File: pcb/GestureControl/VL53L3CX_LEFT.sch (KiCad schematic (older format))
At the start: 25 parts, among them U11 VL53L3CXV0DH_LEFT, U5 VL53L3CXV0DH_LEFT, U9 VL53L3CXV0DH_LEFT

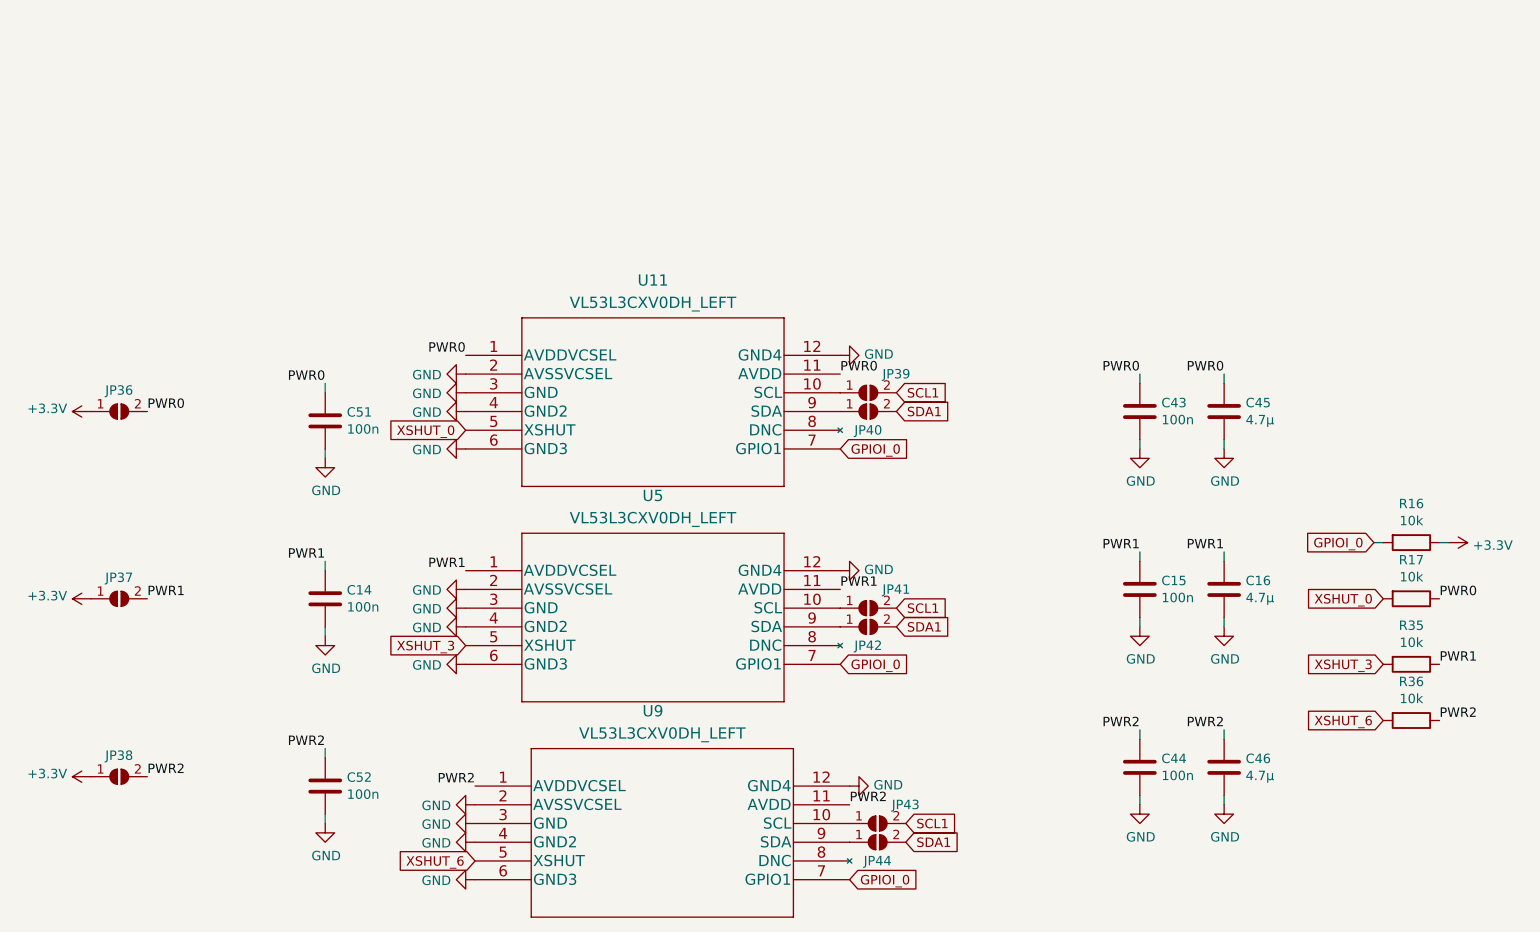
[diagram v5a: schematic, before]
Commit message: add PCB V12
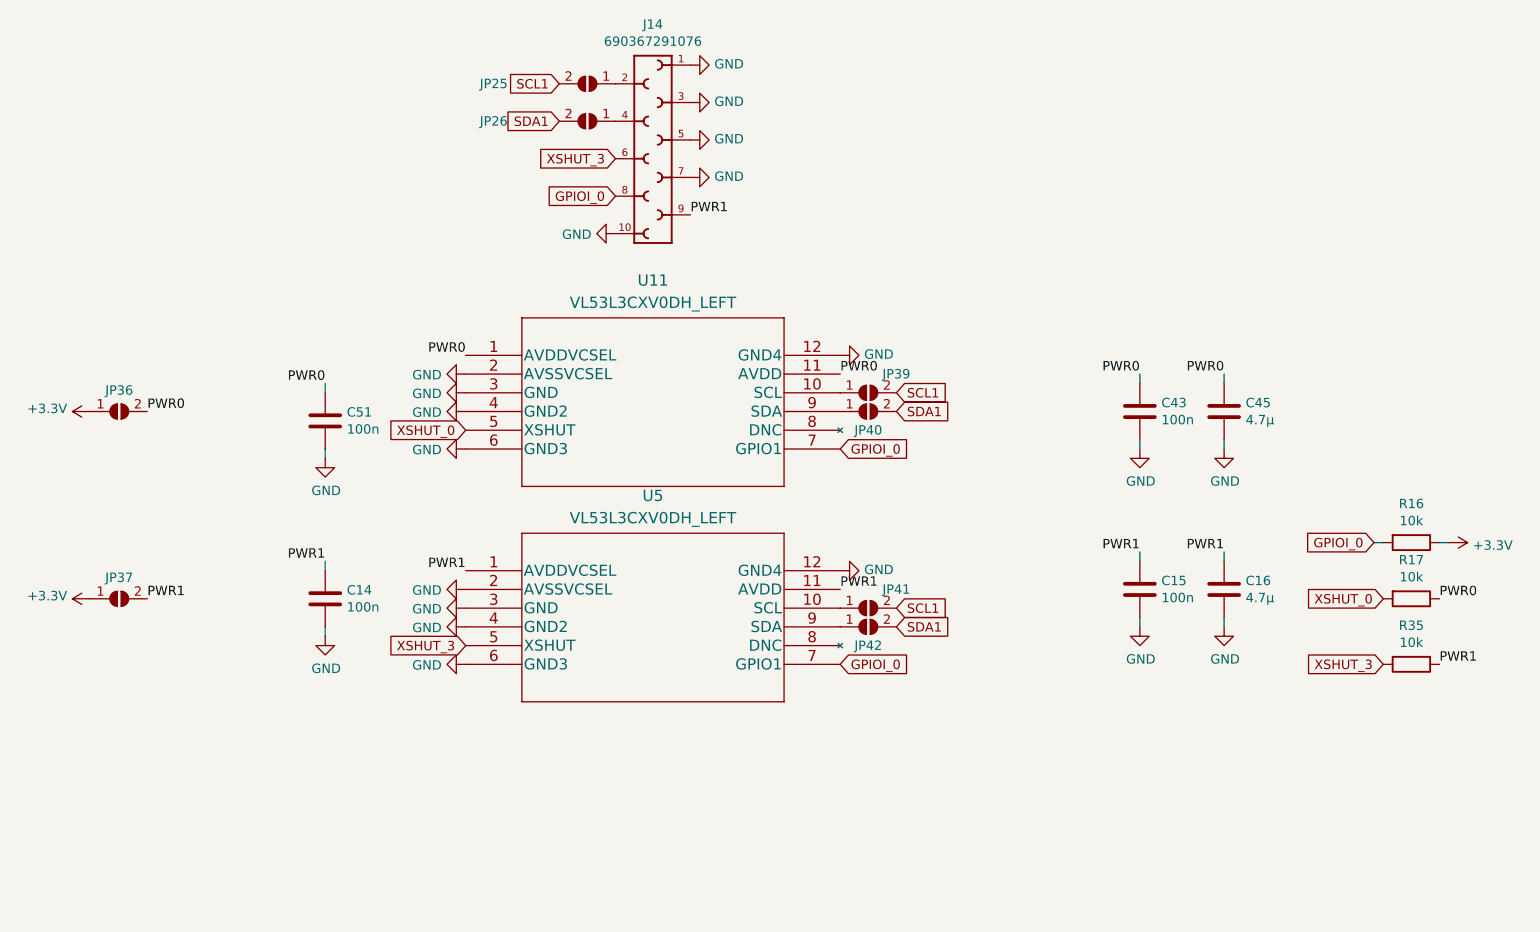
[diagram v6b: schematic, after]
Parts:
- removed C44, C52: 100n, Capacitor_SMD:C_0603_1608Metric_Pad1.08x0.95mm_HandSolder, symbol Device:C
- removed C46: 4.7µ, Capacitor_SMD:C_0805_2012Metric_Pad1.18x1.45mm_HandSolder, symbol Device:C
- removed JP38, JP43, JP44: SolderJumper_2_Open, Jumper:SolderJumper-2_P1.3mm_Open_Pad1.0x1.5mm, symbol Jumper:SolderJumper_2_Open
- removed R36: 10k, Resistor_SMD:R_0805_2012Metric_Pad1.20x1.40mm_HandSolder, symbol Device:R
- removed U9: VL53L3CXV0DH_LEFT, VL53L3CX:VL53L3CXV0DH&slash_1, symbol VL53L3CX:VL53L3CXV0DH_1
- added J14: 690367291076, WR-MM Female SMT Connector:WR-MM Female SMT Connector, symbol WR-MM_Female_SMT_Connector:690367291076
- added JP25, JP26: SolderJumper_2_Open, Jumper:SolderJumper-2_P1.3mm_Open_Pad1.0x1.5mm, symbol Jumper:SolderJumper_2_Open
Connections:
- net GND: now also J14.1, J14.10, J14.3, J14.5, J14.7
- net GPIOI_0: now also J14.8
- net PWR1: now also J14.9
- net SCL1: now also JP25.2 (B)
- net SDA1: now also JP26.2 (B)
- net XSHUT_3: now also J14.6
- new net: J14.4, JP26.1 (A)
- new net: J14.2, JP25.1 (A)
